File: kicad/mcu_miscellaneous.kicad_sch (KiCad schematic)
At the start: 10 parts, among them SW1 SW_Push, SW2 SW_Push

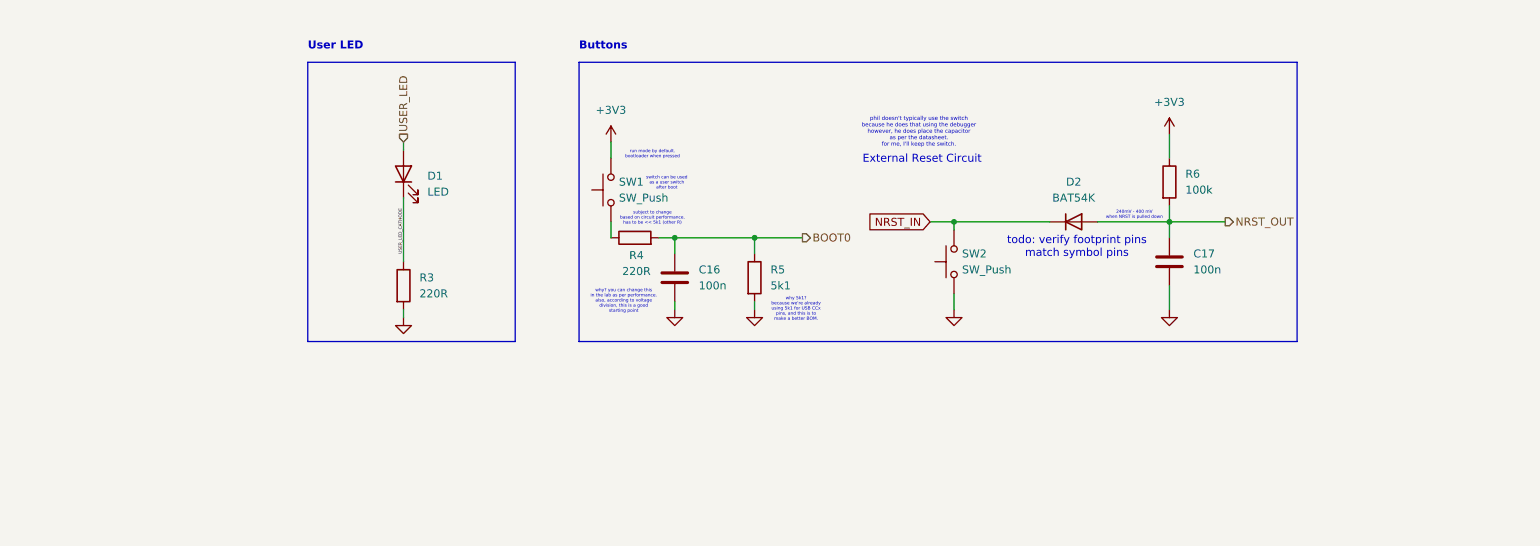
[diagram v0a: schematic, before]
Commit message: everything: select real components, refactor schematic, add a user-led driving circuit, and more
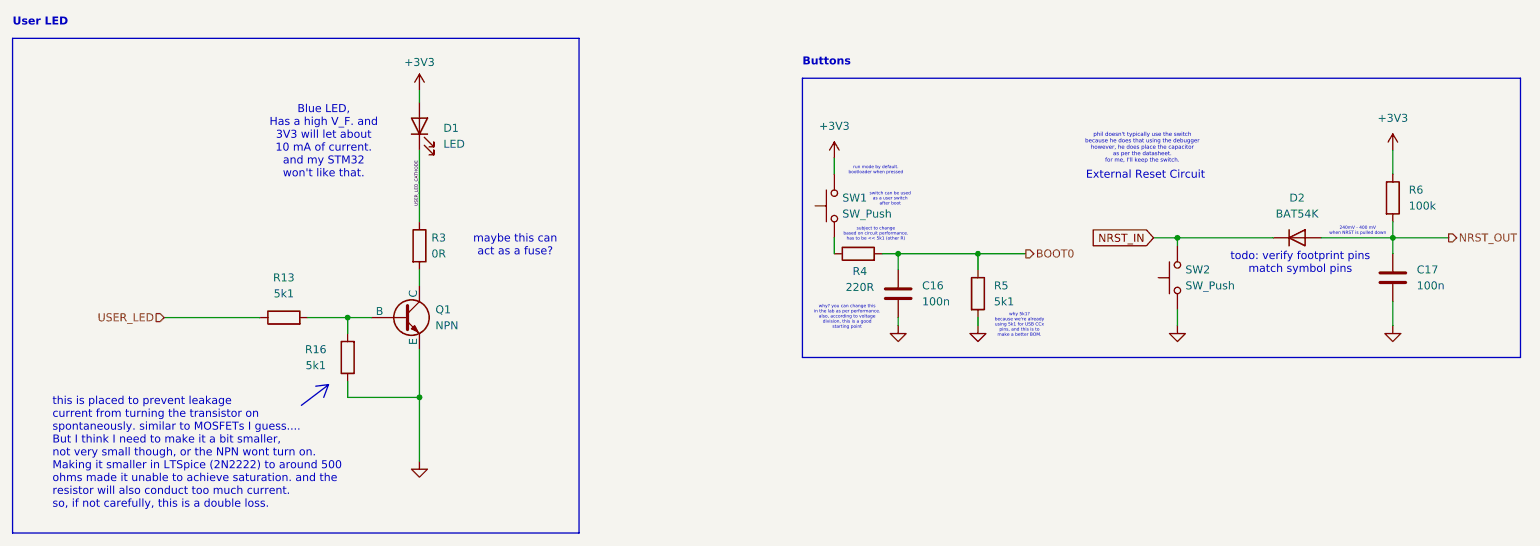
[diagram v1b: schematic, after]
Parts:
- added Q1: NPN, symbol Simulation_SPICE:NPN
- added R13, R16: 5k1, Resistor_SMD:R_0402_1005Metric, symbol Device:R
- C16, C17: footprint (none) -> Capacitor_SMD:C_0402_1005Metric; Distributor (none) -> LCSC; Distributor Link (none) -> https://www.lcsc.com/product-detail/C60474.html?s_z=s_p_CC0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; MPN (none) -> CC0402KRX7R7BB104; Manufacturer (none) -> YAGEO
- D1: footprint (none) -> LED_SMD:LED_0402_1005Metric; Distributor (none) -> LCSC; Distributor Link (none) -> https://www.lcsc.com/product-detail/C511042.html?s_z=s_p_VL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; MPN (none) -> VLMB1500-GS08; Manufacturer (none) -> VISHAY
- D2: Distributor (none) -> LCSC; MPN (none) -> BAT54KFILM; Manufacturer Part Number BAT54KFILM -> (none)
- R3: value 220R -> 0R; footprint (none) -> Resistor_SMD:R_0402_1005Metric
- R4, R5, R6: footprint (none) -> Resistor_SMD:R_0402_1005Metric
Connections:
- net +3V3: now also D1.2 (A)
- net GND: now also Q1.3 (E), R16.1; no longer R3.2
- net USER_LED: now also R13.1; no longer D1.2 (A)
- new net: Q1.1 (C), R3.2
- new net: Q1.2 (B), R13.2, R16.2
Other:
- note added: "Blue LED, Has a high V_F. and 3V3 will let about 10 mA of current. and my STM32 won't like that."
- note added: "maybe this can act as a fuse?"
- note added: "this is placed to prevent leakage current from turning the transistor on spontaneously. similar to MOSFETs I guess.... But I think I need to make it a bit smaller, not very small though, or the NPN wont turn on. Making it smaller in LTSpice (2N2222) to around 500 ohms made it unable to achieve saturation. and the resistor will also conduct too much current. so, if not carefully, this is a double 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"
- moved on the sheet: C16, C17, D1, D2, R3, R4, R5, R6, SW1, SW2
